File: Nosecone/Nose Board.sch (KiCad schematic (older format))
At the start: 51 parts, among them J1 Conn_01x02, J2 Conn_02x04_Odd_Even, J3 Conn_02x03_Odd_Even, J4 Conn_Coaxial, J5 Conn_01x02, Q1 Q_PMOS_DGS, Q2 Q_PMOS_DGS, U1 RS485_converter_ISL83488, U10 MS5803-14BA, U11 MS5803-14BA, U12 Via-stitch, U13 Via-stitch, U14 Via-stitch, U15 Via-stitch, U2 ATXMEGA16A4U-AU, U3 3.3V_DCDC_Conv_TPS62056DGS, U4 GPS_UBX_CAM_M8C, U5 Via-stitch, U6 XBEE, U7 OpenLog, U8 BNO055, U9 LTC4412

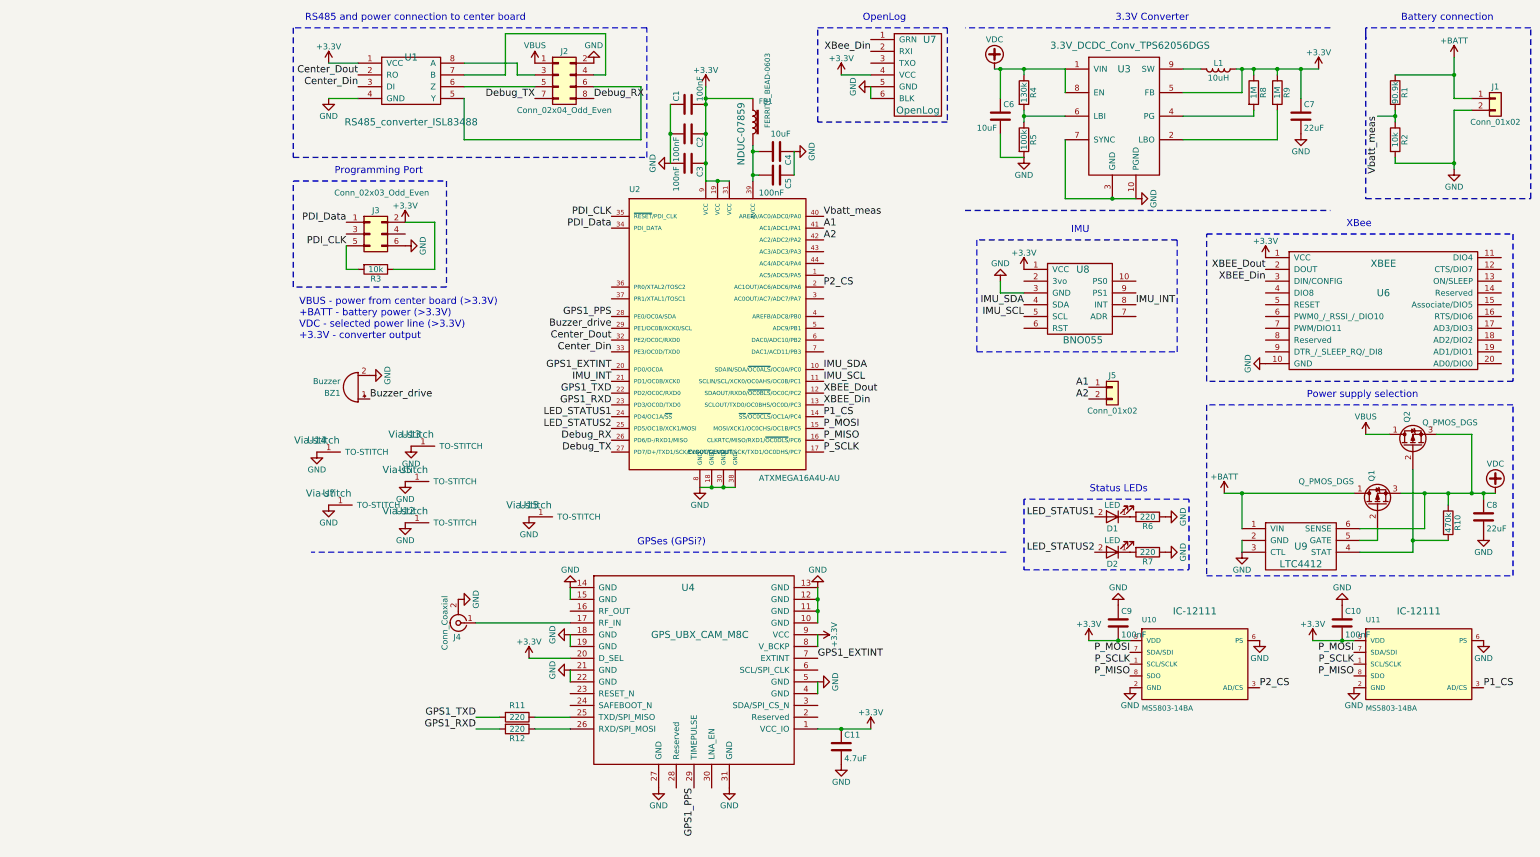
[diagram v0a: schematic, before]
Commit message: Better routing
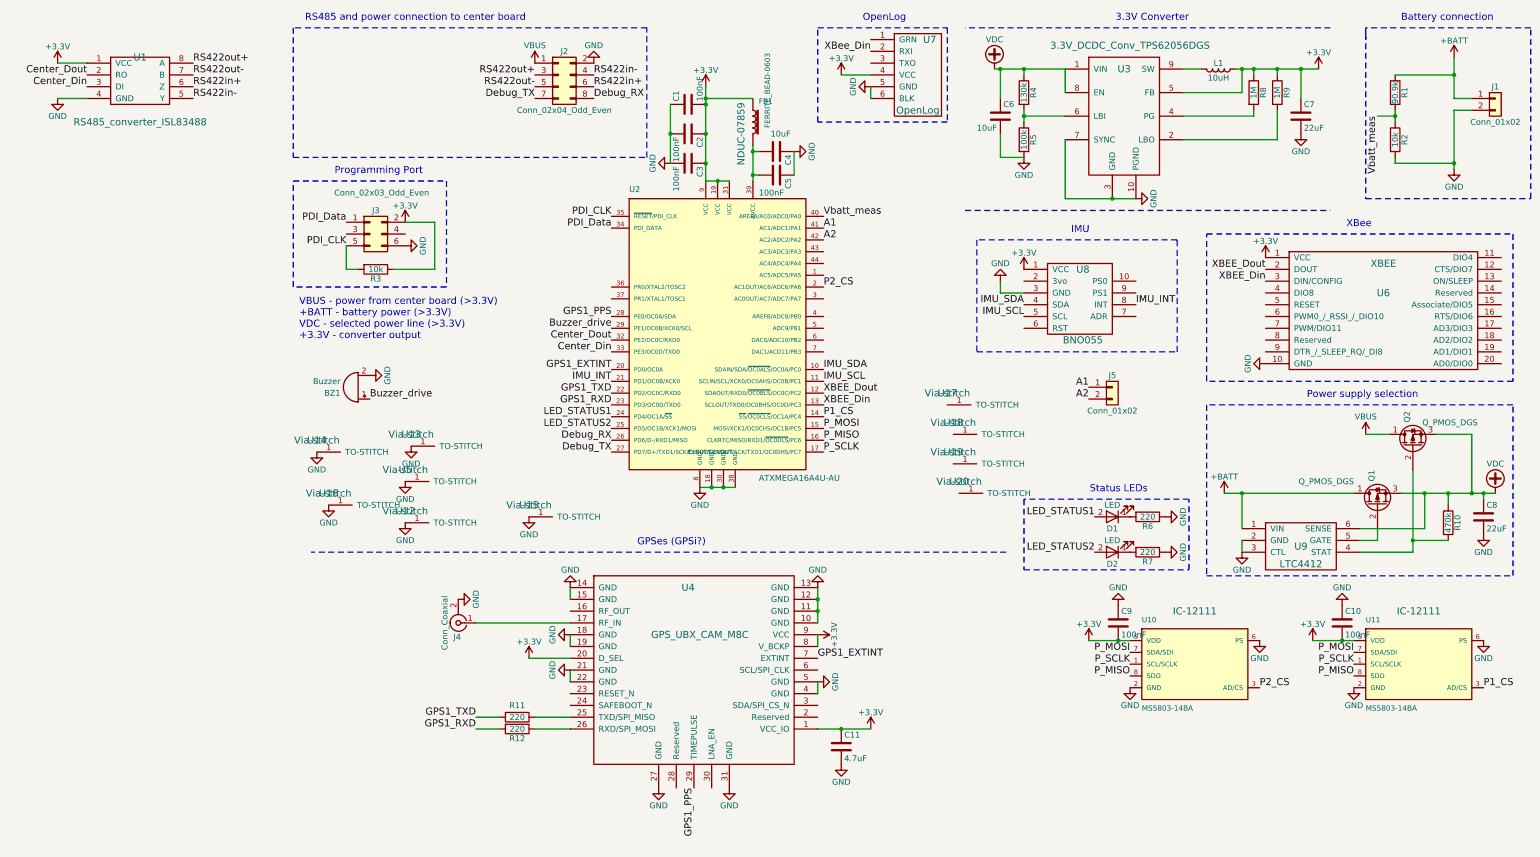
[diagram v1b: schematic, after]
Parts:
- added U17, U18, U19, U20: Via-stitch, Misc components:4_40_through_hole, symbol Via-stitch
- gave numbers to parts that had none: 1
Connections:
- net RS422in+: now reaches J2.6 (Pin_6)
- net RS422in+: now also U1.6 (Z); no longer U1.5 (Y)
- net RS422out-: now reaches J2.5 (Pin_5)
- net RS422out-: now also U1.7 (B); no longer U1.6 (Z)
- net RS422in-: now reaches J2.4 (Pin_4)
- net RS422in-: now also U1.5 (Y); no longer U1.7 (B)
- net RS422out+: now reaches J2.3 (Pin_3), U1.8 (A)
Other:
- moved on the sheet: U1
